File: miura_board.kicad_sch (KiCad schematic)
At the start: 40 parts, among them J1 Screw_Terminal_01x02, J2 Screw_Terminal_01x02, J3 Screw_Terminal_01x02, J4 Conn_01x04_Male, J5 Screw_Terminal_01x02, J6 Screw_Terminal_01x02, J7 Screw_Terminal_01x02, J8 Screw_Terminal_01x02, SW1 SW_Push, SW2 SW_Push, U1 ESP32-WROOM, U3 DRV8833PW, U4 DRV8833PW, U5 AMS1117, U6 MPU-6050, U7 L7806, U8 DRV8833PW

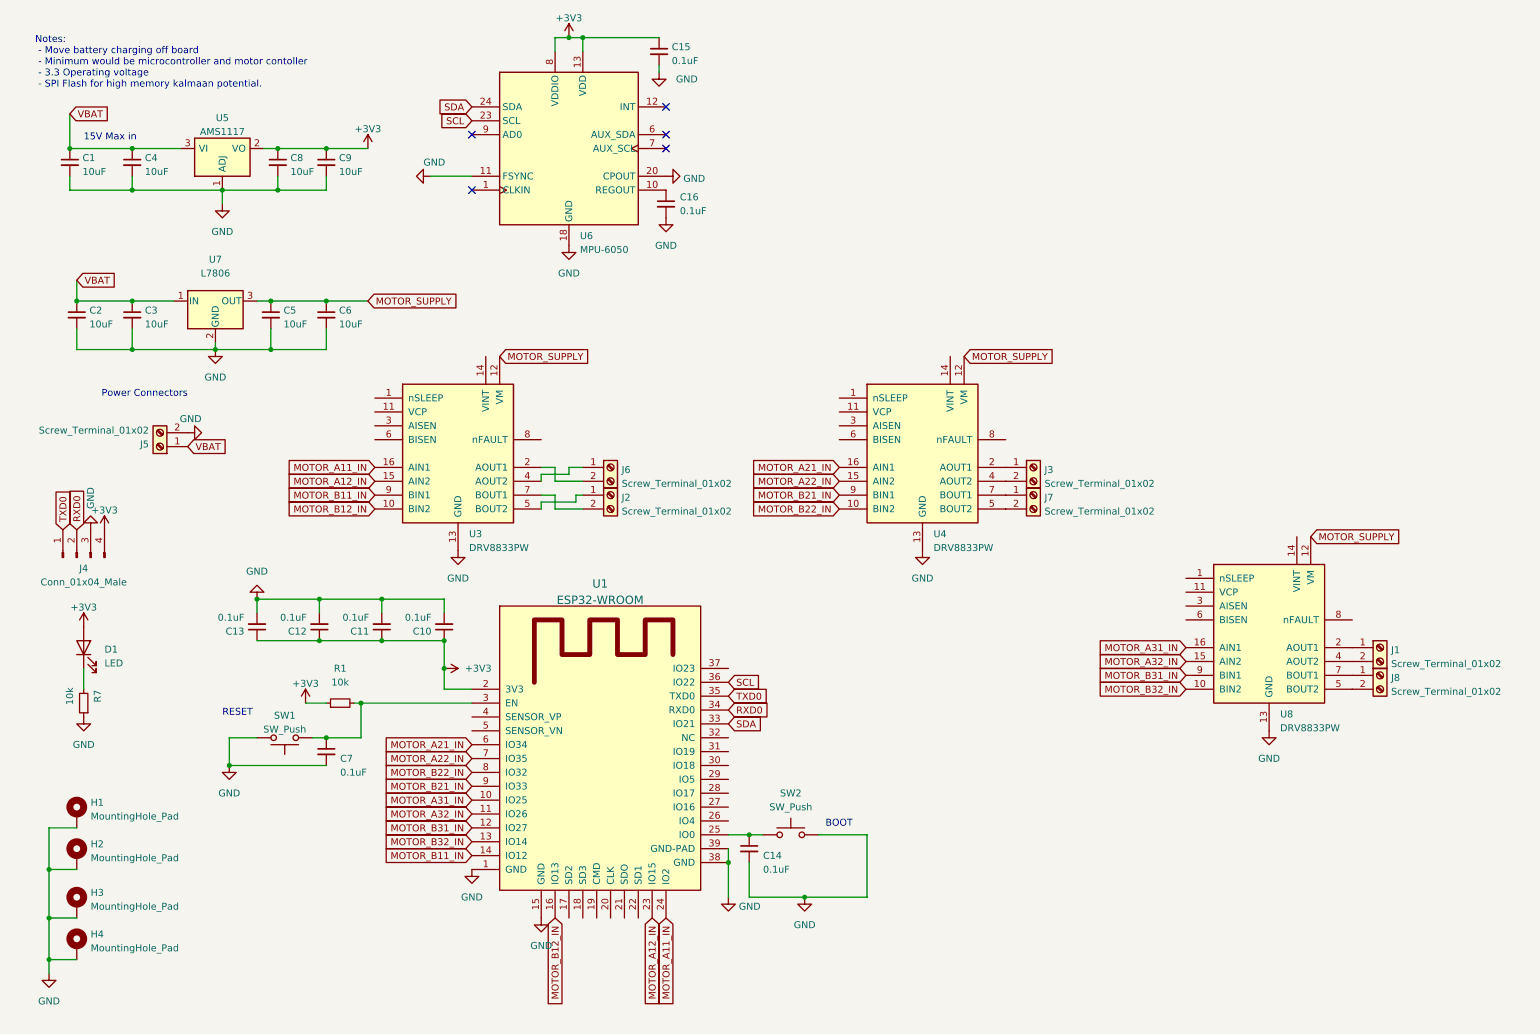
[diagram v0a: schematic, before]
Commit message: Working motor controller
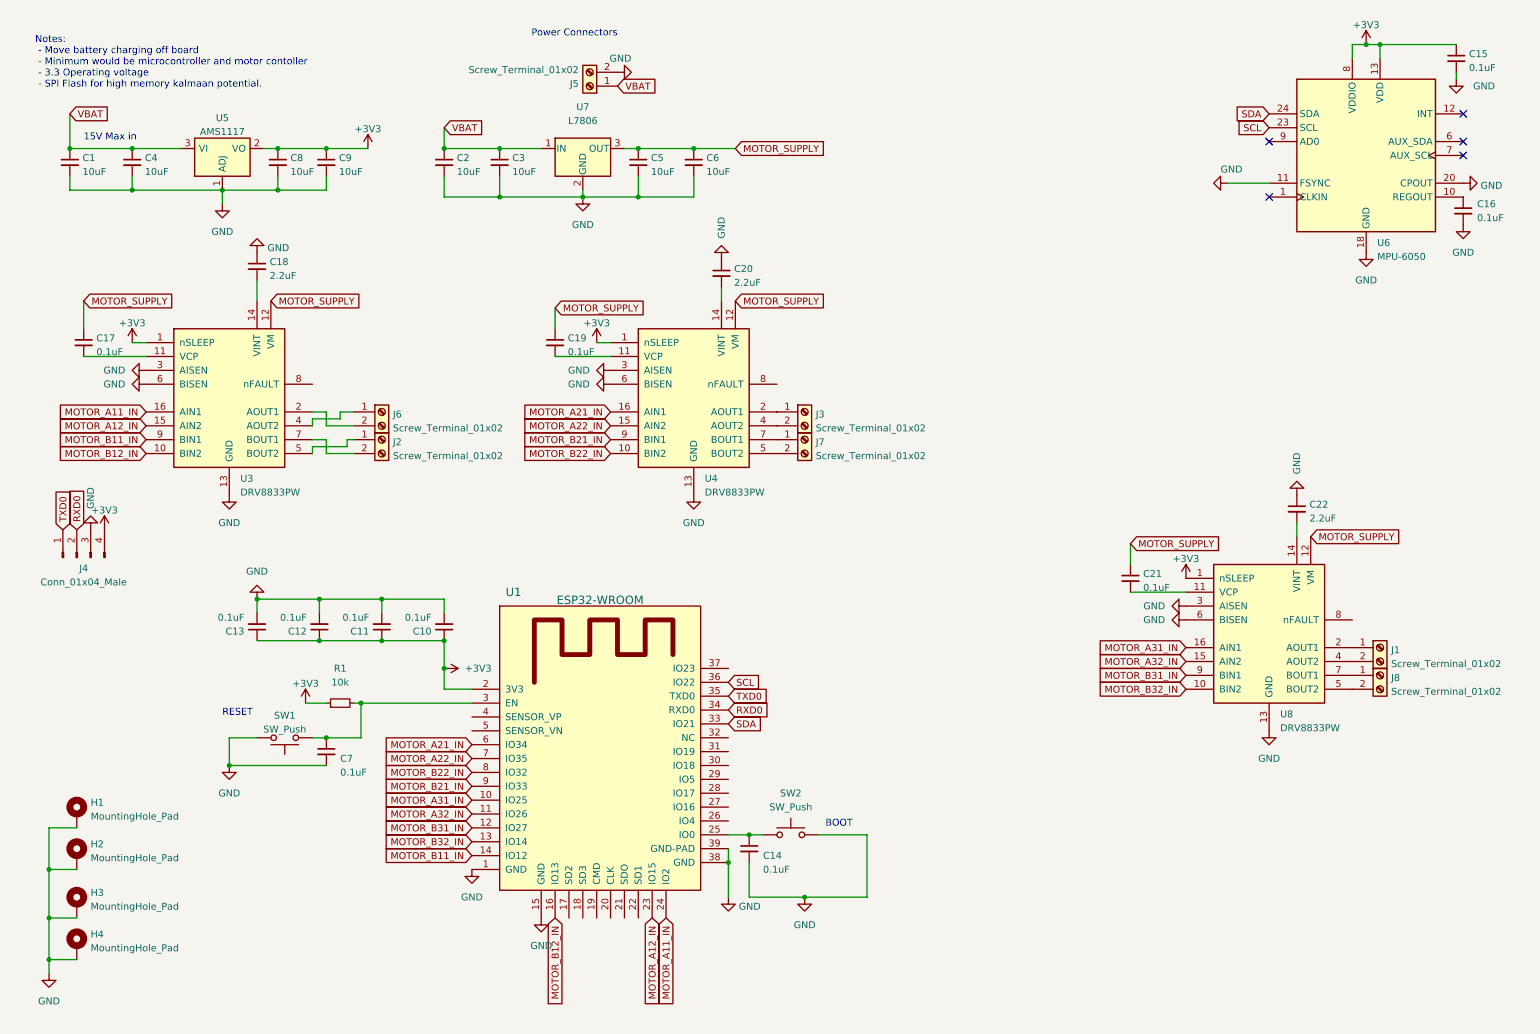
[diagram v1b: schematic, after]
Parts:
- removed D1: LED, LED_SMD:LED_0603_1608Metric, symbol Device:LED
- removed R7: 10k, Resistor_SMD:R_0603_1608Metric_Pad0.98x0.95mm_HandSolder, symbol Device:R_Small
- added C17, C19, C21: 0.1uF, Capacitor_SMD:C_0603_1608Metric, symbol Device:C_Small
- added C18, C20, C22: 2.2uF, Capacitor_SMD:C_0603_1608Metric, symbol Device:C_Small
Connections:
- net +3V3: now also U3.1 (nSLEEP), U4.1 (nSLEEP), U8.1 (nSLEEP)
- net GND: now also U3.3 (AISEN), U3.6 (BISEN), U4.3 (AISEN), U4.6 (BISEN), U8.3 (AISEN), U8.6 (BISEN), C18.1, C20.1, C22.1
- net MOTOR_SUPPLY: now also C17.1, C19.1, C21.1
- net at U3.11 (VCP): now also C17.2
- net at U3.14 (VINT): now also C18.2
- net at U4.11 (VCP): now also C19.2
- net at U4.14 (VINT): now also C20.2
- net at U8.11 (VCP): now also C21.2
- net at U8.14 (VINT): now also C22.2
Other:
- moved on the sheet: C15, C16, C2, C3, C5, C6, J2, J3, J5, J6, J7, U3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

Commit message: new board design
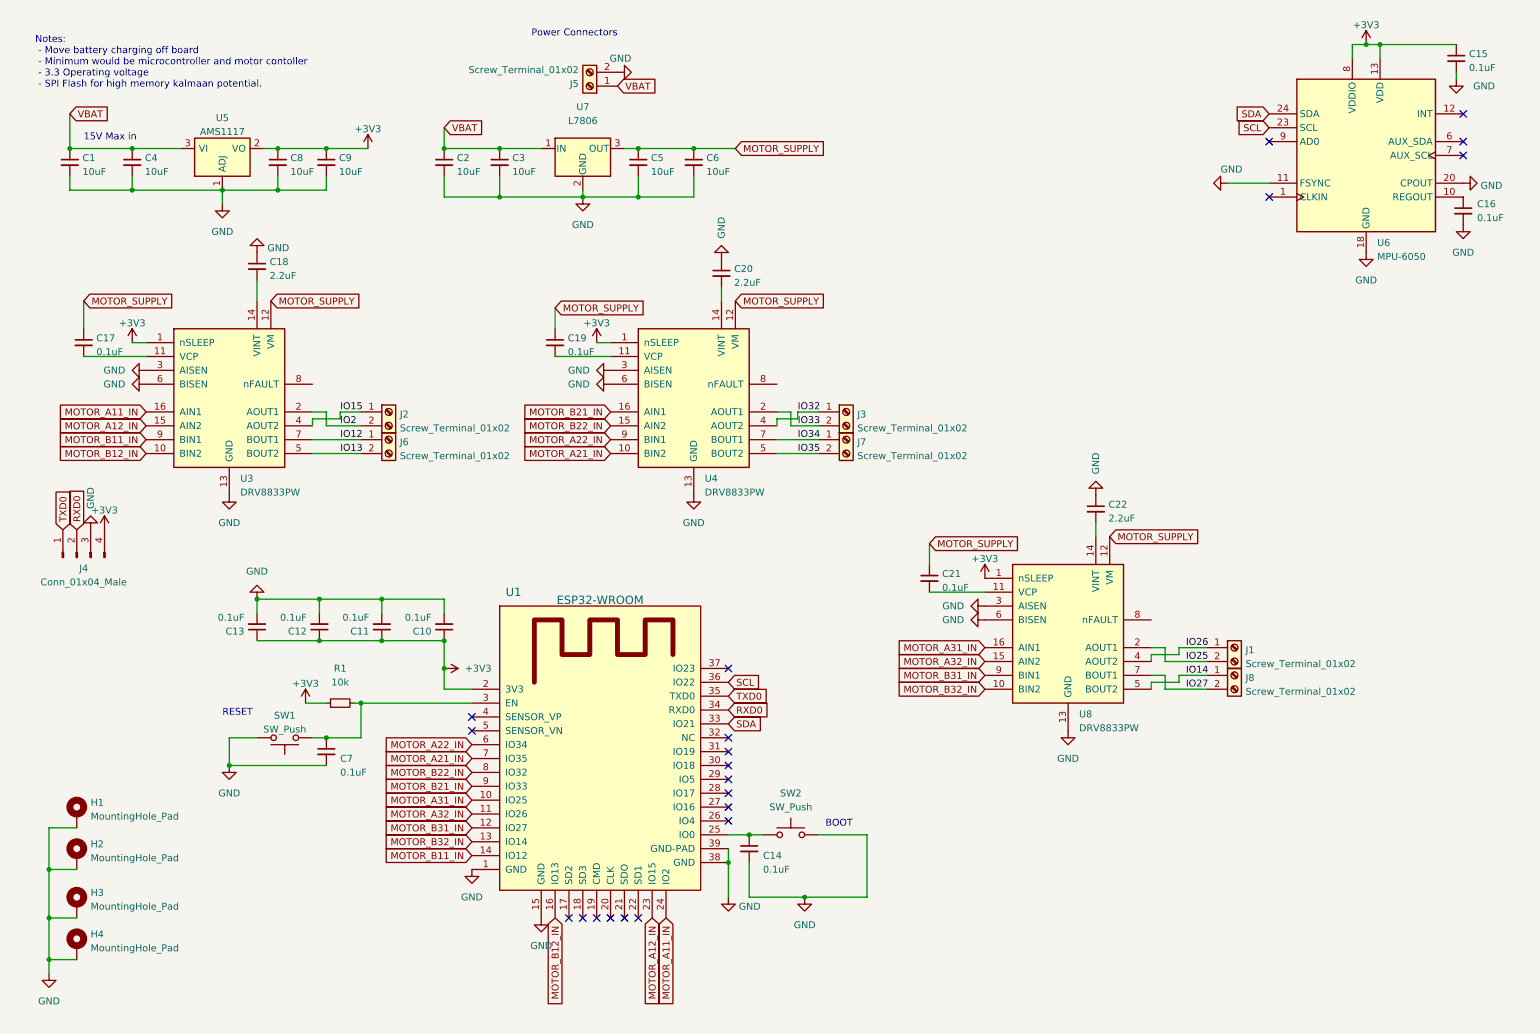
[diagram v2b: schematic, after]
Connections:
- net MOTOR_A21_IN: now also U1.7 (IO35), U4.10 (BIN2); no longer U1.6 (IO34), U4.16 (AIN1)
- net MOTOR_A22_IN: now also U1.6 (IO34), U4.9 (BIN1); no longer U1.7 (IO35), U4.15 (AIN2)
- net MOTOR_B21_IN: now also U4.16 (AIN1); no longer U4.9 (BIN1)
- net MOTOR_B22_IN: now also U4.15 (AIN2); no longer U4.10 (BIN2)
- net IO32: now reaches J3.1 (Pin_1)
- net IO32: now also U4.4 (AOUT2); no longer U4.2 (AOUT1)
- net IO33: now reaches J3.2 (Pin_2)
- net IO33: now also U4.2 (AOUT1); no longer U4.4 (AOUT2)
- net IO25: now reaches U8.2 (AOUT1)
- net IO25: now also J1.2 (Pin_2); no longer J1.1 (Pin_1)
- net IO26: now reaches U8.4 (AOUT2)
- net IO26: now also J1.1 (Pin_1); no longer J1.2 (Pin_2)
- net IO13: now reaches J6.2 (Pin_2)
- net IO13: now also U3.5 (BOUT2); no longer U3.2 (AOUT1)
- net IO12: now reaches J6.1 (Pin_1)
- net IO12: now also U3.7 (BOUT1); no longer U3.4 (AOUT2)
- net IO15: now reaches J2.1 (Pin_1)
- net IO15: now also U3.4 (AOUT2); no longer U3.5 (BOUT2)
- net IO2: now reaches J2.2 (Pin_2)
- net IO2: now also U3.2 (AOUT1); no longer U3.7 (BOUT1)
- net IO35: now reaches J7.2 (Pin_2), U4.5 (BOUT2)
- net IO34: now reaches J7.1 (Pin_1), U4.7 (BOUT1)
- net IO14: now reaches U8.5 (BOUT2)
- net IO14: now also J8.1 (Pin_1); no longer J8.2 (Pin_2)
- net IO27: now reaches U8.7 (BOUT1)
- net IO27: now also J8.2 (Pin_2); no longer J8.1 (Pin_1)
- no-connect marks 5 -> 21
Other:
- moved on the sheet: C21, C22, J1, J2, J3, J6, J7, J8, U8
